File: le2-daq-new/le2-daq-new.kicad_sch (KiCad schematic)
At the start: 23 parts, among them J1 RELAY-CONN, J10 PWR-RAIL, J11 PWR-RAIL, J12 PWR-RAIL, J13 PWR-RAIL, J14 PWR-RAIL, J15 PWR-RAIL, J16 PWR-RAIL, J17 Screw_Terminal_01x02, J2 PT-CONN, J3 TC-CONN, J4 CAP-CONN, J5 PWR-RAIL, J6 PWR-RAIL, J7 PWR-RAIL, J8 PWR-RAIL, J9 PWR-RAIL, U1 ESP32-DEVKITC-32D

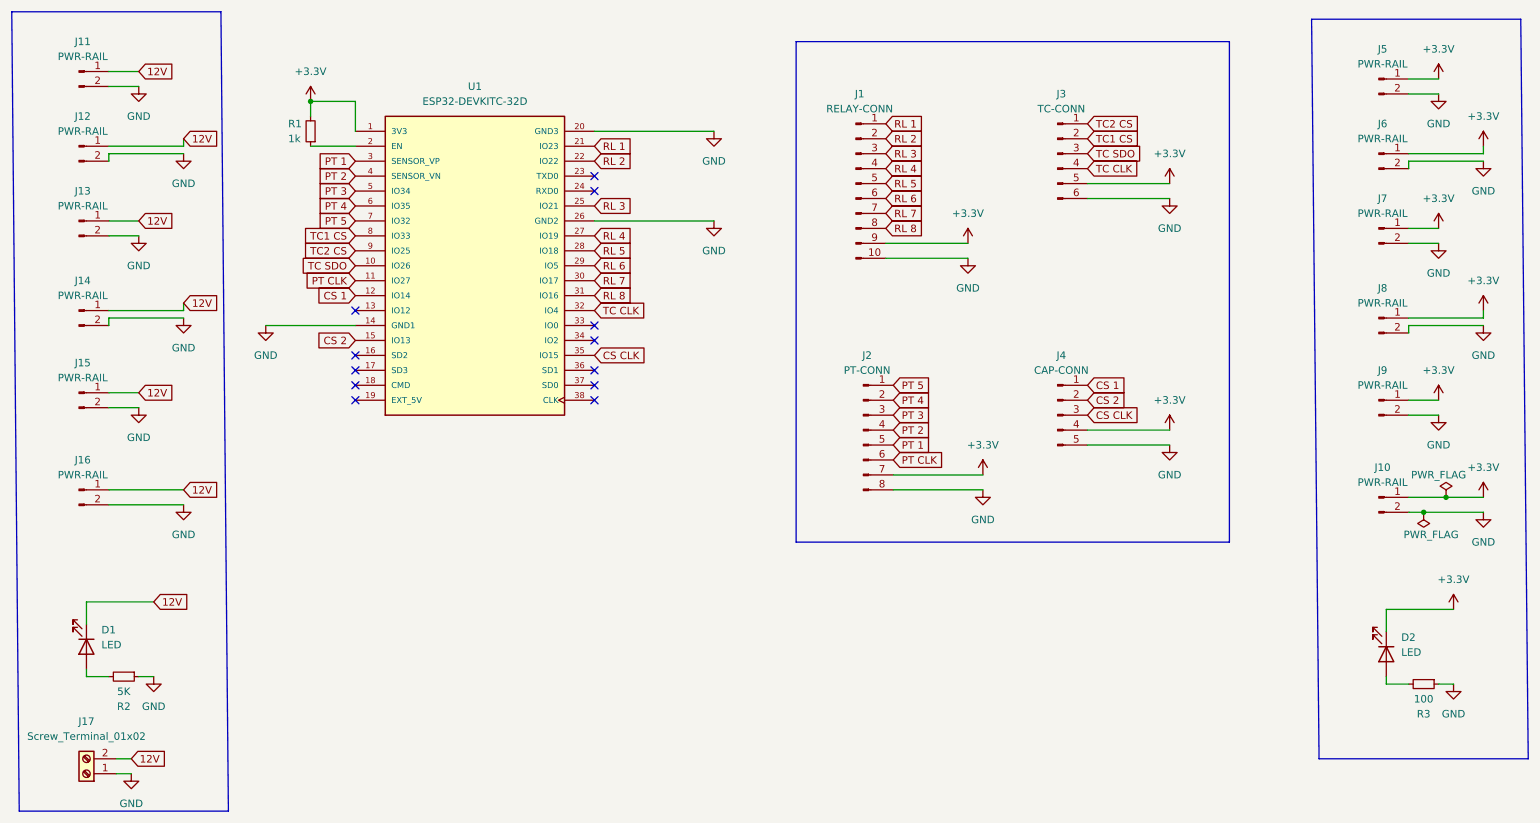
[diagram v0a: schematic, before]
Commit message: stash
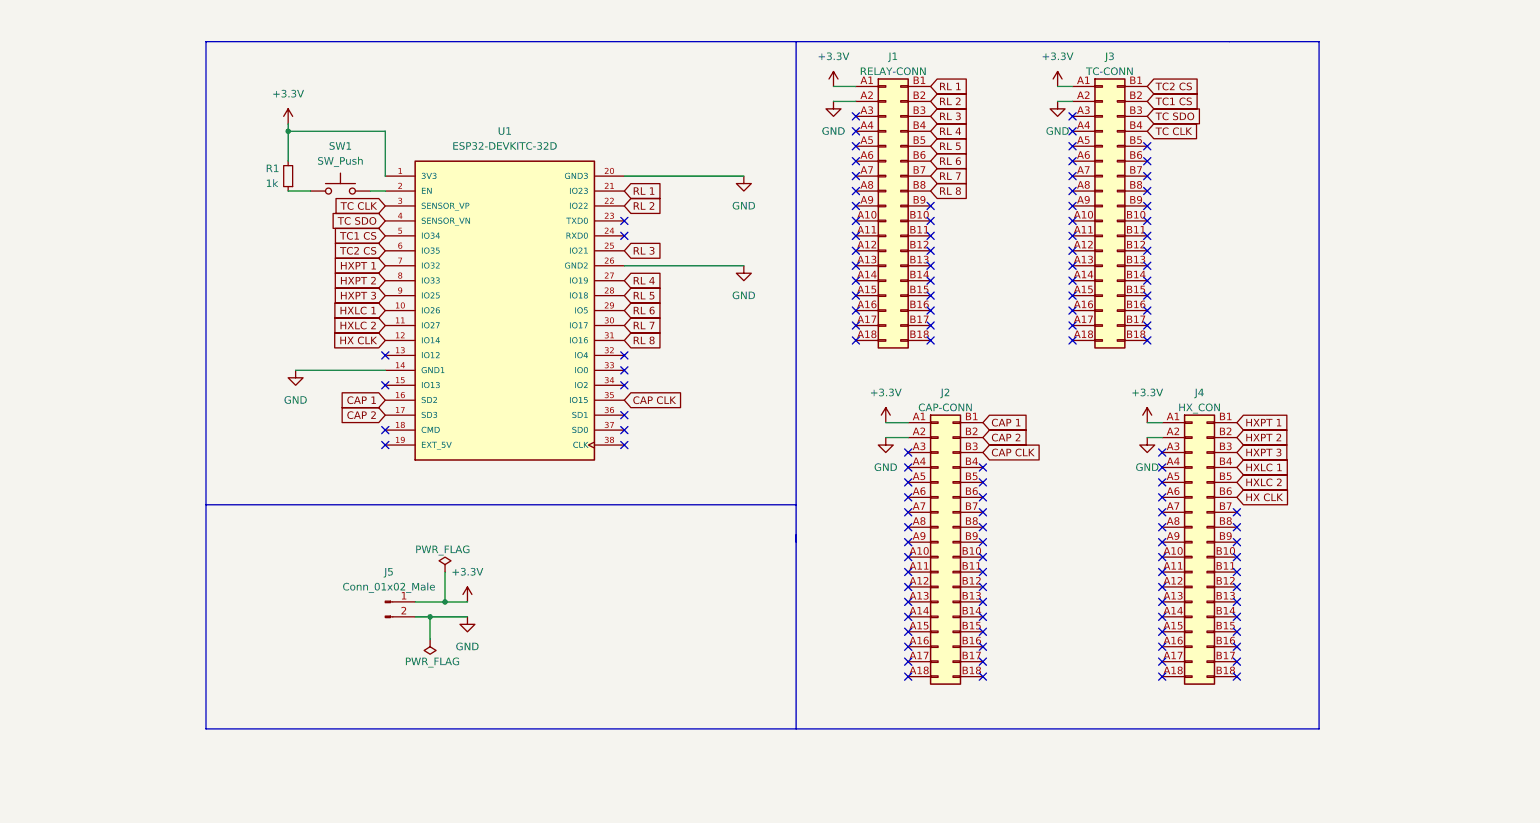
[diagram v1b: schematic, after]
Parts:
- removed D1, D2: LED, LED_THT:LED_D3.0mm, symbol Device:LED
- removed J10, J11, J12, J13, J14, J15, J16, J6, J7, J8, J9: PWR-RAIL, Connector_PinHeader_2.54mm:PinHeader_1x02_P2.54mm_Horizontal, symbol Connector:Conn_01x02_Male
- removed J17: Screw_Terminal_01x02, Connector_PinHeader_2.54mm:PinHeader_1x02_P2.54mm_Horizontal, symbol Connector:Screw_Terminal_01x02
- removed J2: PT-CONN, Connector_PinHeader_2.54mm:PinHeader_1x09_P2.54mm_Horizontal, symbol Connector:Conn_01x08_Male
- removed J3: TC-CONN, Connector_PinHeader_2.54mm:PinHeader_1x06_P2.54mm_Horizontal, symbol Connector:Conn_01x06_Male
- removed J4: CAP-CONN, Connector_PinHeader_2.54mm:PinHeader_1x05_P2.54mm_Horizontal, symbol Connector:Conn_01x05_Male
- removed R2: 5K, Resistor_SMD:R_0805_2012Metric_Pad1.20x1.40mm_HandSolder, symbol Device:R_Small
- removed R3: 100, Resistor_SMD:R_0805_2012Metric_Pad1.20x1.40mm_HandSolder, symbol Device:R_Small
- added J2: CAP-CONN, PCIE_1x_Socket:AMPHENOL_10018784-10210TLF, symbol Connector_Generic:Conn_02x18_Row_Letter_First
- added J3: TC-CONN, PCIE_1x_Socket:AMPHENOL_10018784-10210TLF, symbol Connector_Generic:Conn_02x18_Row_Letter_First
- added J4: HX_CON, PCIE_1x_Socket:AMPHENOL_10018784-10210TLF, symbol Connector_Generic:Conn_02x18_Row_Letter_First
- added SW1: SW_Push, Jumper:SolderJumper-2_P1.3mm_Bridged2Bar_Pad1.0x1.5mm, symbol Switch:SW_Push
- J1: footprint Connector_PinHeader_2.54mm:PinHeader_1x10_P2.54mm_Horizontal -> PCIE_1x_Socket:AMPHENOL_10018784-10210TLF; symbol Connector:Conn_01x10_Male -> Connector_Generic:Conn_02x18_Row_Letter_First
- J5: value PWR-RAIL -> Conn_01x02_Male
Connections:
- net PT 1 is gone; now on net TC CLK: U1.3 (SENSOR_VP)
- net PT 2 is gone; now on net TC SDO: U1.4 (SENSOR_VN)
- net PT 3 is gone; now on net TC1 CS: U1.5 (IO34)
- net PT 4 is gone; now on net TC2 CS: U1.6 (IO35)
- net +3.3V: now also J1.A1 (Pin_a1), J2.A1 (Pin_a1), J3.A1 (Pin_a1), J4.A1 (Pin_a1); no longer J1.9 (Pin_9)
- net GND: now also J1.A2 (Pin_a2), J2.A2 (Pin_a2), J3.A2 (Pin_a2), J4.A2 (Pin_a2); no longer J1.10 (Pin_10)
- net RL 1: now also J1.B1 (Pin_b1); no longer J1.1 (Pin_1)
- net RL 2: now also J1.B2 (Pin_b2); no longer J1.2 (Pin_2)
- net RL 3: now also J1.B3 (Pin_b3); no longer J1.3 (Pin_3)
- net RL 4: now also J1.B4 (Pin_b4); no longer J1.4 (Pin_4)
- net RL 5: now also J1.B5 (Pin_b5); no longer J1.5 (Pin_5)
- net RL 6: now also J1.B6 (Pin_b6); no longer J1.6 (Pin_6)
- net RL 7: now also J1.B7 (Pin_b7); no longer J1.7 (Pin_7)
- net RL 8: now also J1.B8 (Pin_b8); no longer J1.8 (Pin_8)
- net TC CLK: now also J3.B4 (Pin_b4); no longer U1.32 (IO4)
- net TC SDO: now also J3.B3 (Pin_b3); no longer U1.10 (IO26)
- net TC1 CS: now also J3.B2 (Pin_b2); no longer U1.8 (IO33)
- net TC2 CS: now also J3.B1 (Pin_b1); no longer U1.9 (IO25)
- net at R1.1: now also SW1.1; no longer U1.2 (EN)
- net CAP 1: now reaches U1.16 (SD2)
- net CAP 1: now also J2.B1 (Pin_b1)
- net CAP 2: now reaches U1.17 (SD3)
- net CAP 2: now also J2.B2 (Pin_b2)
- net CS 1 renamed HX CLK
- net HX CLK: now also J4.B6 (Pin_b6)
- net CS 2: no longer names the net of U1.15 (IO13)
- net CS CLK renamed CAP CLK
- net CAP CLK: now also J2.B3 (Pin_b3)
- net PT 5 renamed HXPT 1
- net HXPT 1: now also J4.B1 (Pin_b1)
- net PT CLK renamed HXLC 2
- net HXLC 2: now also J4.B5 (Pin_b5)
- new net: SW1.2, U1.2 (EN)
- new net HXLC 1: J4.B4 (Pin_b4), U1.10 (IO26)
- new net HXPT 2: J4.B2 (Pin_b2), U1.8 (IO33)
- new net HXPT 3: J4.B3 (Pin_b3), U1.9 (IO25)
- no-connect marks 12 -> 127
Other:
- moved on the sheet: R1, U1

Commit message: CORE PCB DONE
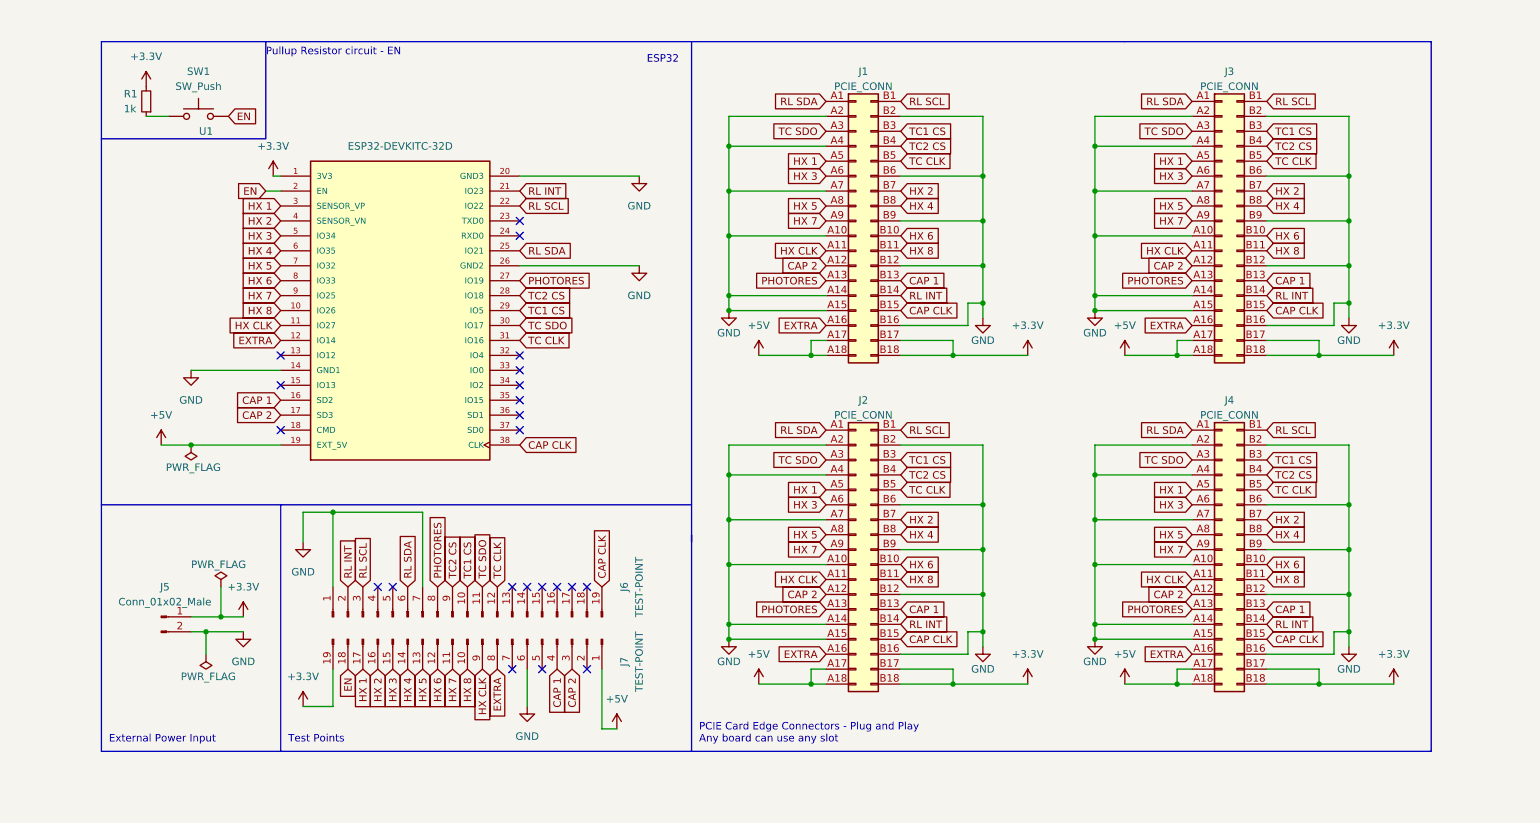
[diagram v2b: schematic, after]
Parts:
- added J6, J7: TEST-POINT, Connector_PinHeader_2.54mm:PinHeader_1x19_P2.54mm_Horizontal, symbol Connector:Conn_01x19_Male
- J1: value RELAY-CONN -> PCIE_CONN; footprint PCIE_1x_Socket:AMPHENOL_10018784-10210TLF -> PCIE-LP-01-01-F-DV-A-TR:SAMTEC_PCIE-LP-01-01-F-DV-A-TR
- J2: value CAP-CONN -> PCIE_CONN; footprint PCIE_1x_Socket:AMPHENOL_10018784-10210TLF -> PCIE-LP-01-01-F-DV-A-TR:SAMTEC_PCIE-LP-01-01-F-DV-A-TR
- J3: value TC-CONN -> PCIE_CONN; footprint PCIE_1x_Socket:AMPHENOL_10018784-10210TLF -> PCIE-LP-01-01-F-DV-A-TR:SAMTEC_PCIE-LP-01-01-F-DV-A-TR
- J4: value HX_CON -> PCIE_CONN; footprint PCIE_1x_Socket:AMPHENOL_10018784-10210TLF -> PCIE-LP-01-01-F-DV-A-TR:SAMTEC_PCIE-LP-01-01-F-DV-A-TR
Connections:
- net +3.3V: now also J1.B17 (Pin_b17), J1.B18 (Pin_b18), J2.B17 (Pin_b17), J2.B18 (Pin_b18), J3.B17 (Pin_b17), J3.B18 (Pin_b18), J4.B17 (Pin_b17), J4.B18 (Pin_b18), J7.19 (Pin_19); no longer J1.A1 (Pin_a1), J2.A1 (Pin_a1), J3.A1 (Pin_a1), J4.A1 (Pin_a1)
- net CAP 1: now also J1.B13 (Pin_b13), J2.B13 (Pin_b13), J3.B13 (Pin_b13), J4.B13 (Pin_b13), J7.4 (Pin_4); no longer J2.B1 (Pin_b1)
- net CAP 2: now also J1.A12 (Pin_a12), J2.A12 (Pin_a12), J3.A12 (Pin_a12), J4.A12 (Pin_a12), J7.3 (Pin_3); no longer J2.B2 (Pin_b2)
- net CAP CLK: now also J1.B15 (Pin_b15), J2.B15 (Pin_b15), J3.B15 (Pin_b15), J4.B15 (Pin_b15), U1.38 (CLK), J6.19 (Pin_19); no longer J2.B3 (Pin_b3), U1.35 (IO15)
- net GND: now also J1.A10 (Pin_a10), J1.A14 (Pin_a14), J1.A15 (Pin_a15), J1.A4 (Pin_a4), J1.A7 (Pin_a7), J1.B12 (Pin_b12), J1.B16 (Pin_b16), J1.B2 (Pin_b2), J1.B6 (Pin_b6), J1.B9 (Pin_b9), J2.A10 (Pin_a10), J2.A14 (Pin_a14), J2.A15 (Pin_a15), J2.A4 (Pin_a4), J2.A7 (Pin_a7), J2.B12 (Pin_b12), J2.B16 (Pin_b16), J2.B2 (Pin_b2), J2.B6 (Pin_b6), J2.B9 (Pin_b9), J3.A10 (Pin_a10), J3.A14 (Pin_a14), J3.A15 (Pin_a15), J3.A4 (Pin_a4), J3.A7 (Pin_a7), J3.B12 (Pin_b12), J3.B16 (Pin_b16), J3.B2 (Pin_b2), J3.B6 (Pin_b6), J3.B9 (Pin_b9), J4.A10 (Pin_a10), J4.A14 (Pin_a14), J4.A15 (Pin_a15), J4.A4 (Pin_a4), J4.A7 (Pin_a7), J4.B12 (Pin_b12), J4.B16 (Pin_b16), J4.B2 (Pin_b2), J4.B6 (Pin_b6), J4.B9 (Pin_b9), J6.1 (Pin_1), J6.7 (Pin_7), J7.6 (Pin_6)
- net HX CLK: now also J1.A11 (Pin_a11), J2.A11 (Pin_a11), J3.A11 (Pin_a11), J4.A11 (Pin_a11), U1.11 (IO27), J7.9 (Pin_9); no longer J4.B6 (Pin_b6), U1.12 (IO14)
- net TC CLK: now also J1.B5 (Pin_b5), J2.B5 (Pin_b5), J3.B5 (Pin_b5), J4.B5 (Pin_b5), U1.31 (IO16), J6.12 (Pin_12); no longer J3.B4 (Pin_b4), U1.3 (SENSOR_VP)
- net TC SDO: now also J1.A3 (Pin_a3), J2.A3 (Pin_a3), J3.A3 (Pin_a3), J4.A3 (Pin_a3), U1.30 (IO17), J6.11 (Pin_11); no longer J3.B3 (Pin_b3), U1.4 (SENSOR_VN)
- net TC1 CS: now also J1.B3 (Pin_b3), J2.B3 (Pin_b3), J3.B3 (Pin_b3), J4.B3 (Pin_b3), U1.29 (IO5), J6.10 (Pin_10); no longer J3.B2 (Pin_b2), U1.5 (IO34)
- net TC2 CS: now also J1.B4 (Pin_b4), J2.B4 (Pin_b4), J3.B4 (Pin_b4), J4.B4 (Pin_b4), U1.28 (IO18), J6.9 (Pin_9); no longer J3.B1 (Pin_b1), U1.6 (IO35)
- net +5V: now reaches U1.19 (EXT_5V)
- net +5V: now also J1.A17 (Pin_a17), J1.A18 (Pin_a18), J2.A17 (Pin_a17), J2.A18 (Pin_a18), J3.A17 (Pin_a17), J3.A18 (Pin_a18), J4.A17 (Pin_a17), J4.A18 (Pin_a18), J7.1 (Pin_1)
- net EN: now reaches SW1.2, U1.2 (EN)
- net EN: now also J7.18 (Pin_18)
- net PHOTORES: now reaches J3.A13 (Pin_a13)
- net PHOTORES: now also J1.A13 (Pin_a13), J2.A13 (Pin_a13), J4.A13 (Pin_a13), U1.27 (IO19), J6.8 (Pin_8)
- net EXTRA: now reaches J3.A16 (Pin_a16)
- net EXTRA: now also J1.A16 (Pin_a16), J2.A16 (Pin_a16), J4.A16 (Pin_a16), U1.12 (IO14), J7.8 (Pin_8)
- net HX 1: now reaches J3.A5 (Pin_a5)
- net HX 1: now also J1.A5 (Pin_a5), J2.A5 (Pin_a5), J4.A5 (Pin_a5), U1.3 (SENSOR_VP), J7.17 (Pin_17)
- net HX 3: now reaches J3.A6 (Pin_a6)
- net HX 3: now also J1.A6 (Pin_a6), J2.A6 (Pin_a6), J4.A6 (Pin_a6), U1.5 (IO34), J7.15 (Pin_15)
- net HX 5: now reaches J3.A8 (Pin_a8)
- net HX 5: now also J1.A8 (Pin_a8), J2.A8 (Pin_a8), J4.A8 (Pin_a8), U1.7 (IO32), J7.13 (Pin_13)
- net HX 7: now reaches J3.A9 (Pin_a9)
- net HX 7: now also J1.A9 (Pin_a9), J2.A9 (Pin_a9), J4.A9 (Pin_a9), U1.9 (IO25), J7.11 (Pin_11)
- net HX 6: now reaches J3.B10 (Pin_b10)
- net HX 6: now also J1.B10 (Pin_b10), J2.B10 (Pin_b10), J4.B10 (Pin_b10), U1.8 (IO33), J7.12 (Pin_12)
- net HX 8: now reaches J3.B11 (Pin_b11)
- net HX 8: now also J1.B11 (Pin_b11), J2.B11 (Pin_b11), J4.B11 (Pin_b11), U1.10 (IO26), J7.10 (Pin_10)
- net RL INT: now reaches J3.B14 (Pin_b14)
- net RL INT: now also J1.B14 (Pin_b14), J2.B14 (Pin_b14), J4.B14 (Pin_b14), U1.21 (IO23), J6.2 (Pin_2)
- net HX 2: now reaches J3.B7 (Pin_b7)
- net HX 2: now also J1.B7 (Pin_b7), J2.B7 (Pin_b7), J4.B7 (Pin_b7), U1.4 (SENSOR_VN), J7.16 (Pin_16)
- net HX 4: now reaches J3.B8 (Pin_b8)
- net HX 4: now also J1.B8 (Pin_b8), J2.B8 (Pin_b8), J4.B8 (Pin_b8), U1.6 (IO35), J7.14 (Pin_14)
- removed net HXLC 1: J4.B4 (Pin_b4), U1.10 (IO26)
- removed net HXLC 2: J4.B5 (Pin_b5), U1.11 (IO27)
- net HXPT 1 renamed RL SCL
- net RL SCL: now also J1.B1 (Pin_b1), J2.B1 (Pin_b1), J3.B1 (Pin_b1), U1.22 (IO22), J6.3 (Pin_3); no longer U1.7 (IO32)
- removed net HXPT 2: J4.B2 (Pin_b2), U1.8 (IO33)
- removed net HXPT 3: J4.B3 (Pin_b3), U1.9 (IO25)
- removed net RL 1: J1.B1 (Pin_b1), U1.21 (IO23)
- removed net RL 2: J1.B2 (Pin_b2), U1.22 (IO22)
- net RL 3 renamed RL SDA
- net RL SDA: now also J1.A1 (Pin_a1), J2.A1 (Pin_a1), J3.A1 (Pin_a1), J4.A1 (Pin_a1), J6.6 (Pin_6); no longer J1.B3 (Pin_b3)
- removed net RL 4: J1.B4 (Pin_b4), U1.27 (IO19)
- removed net RL 5: J1.B5 (Pin_b5), U1.28 (IO18)
- removed net RL 6: J1.B6 (Pin_b6), U1.29 (IO5)
- removed net RL 7: J1.B7 (Pin_b7), U1.30 (IO17)
- removed net RL 8: J1.B8 (Pin_b8), U1.31 (IO16)
- no-connect marks 127 -> 22
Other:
- note added: "ESP32"
- note added: "External Power Input"
- note added: "PCIE Card Edge Connectors - Plug and Play Any board can use any slot"
- note added: "Pullup Resistor circuit - EN"
- note added: "Test Points"
- moved on the sheet: J1, J5, U1
